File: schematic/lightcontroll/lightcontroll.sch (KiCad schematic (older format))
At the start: 0 parts

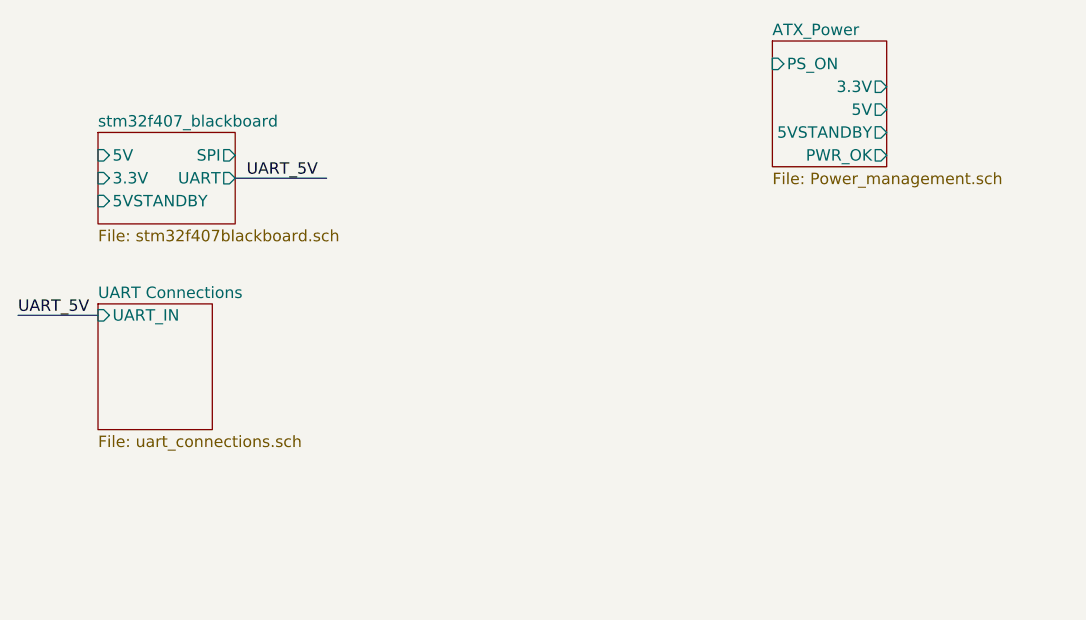
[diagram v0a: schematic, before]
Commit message: build backup
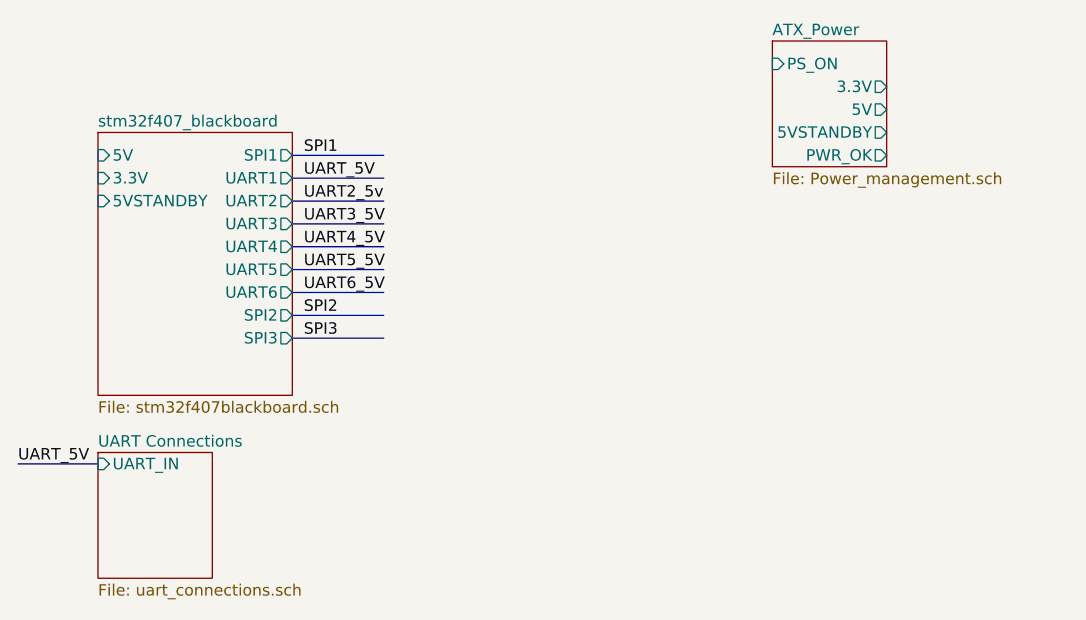
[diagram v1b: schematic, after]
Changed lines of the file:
@@
 $EndDescr
 $Sheet
-S 1600 1350 600  400
+S 1600 1350 850  1150
 U 5C818DF2
 F0 "stm32f407_blackboard" 50
@@
 F3 "3.3V" I L 1600 1550 50
 F4 "5VSTANDBY" I L 1600 1650 50
-F5 "SPI" O R 2200 1450 50
-F6 "UART" O R 2200 1550 50
+F5 "SPI1" O R 2450 1450 50
+F6 "UART1" O R 2450 1550 50
+F7 "UART2" O R 2450 1650 50
+F8 "UART3" O R 2450 1750 50
+F9 "UART4" O R 2450 1850 50
+F10 "UART5" O R 2450 1950 50
+F11 "UART6" O R 2450 2050 50
+F12 "SPI2" O R 2450 2150 50
+F13 "SPI3" O R 2450 2250 50
 $EndSheet
 $Sheet
@@
 $EndSheet
 $Sheet
-S 1600 2100 500  550
+S 1600 2750 500  550
 U 5C906D74
 F0 "UART Connections" 50
 F1 "uart_connections.sch" 50
-F2 "UART_IN" I L 1600 2150 50
+F2 "UART_IN" I L 1600 2800 50
 $EndSheet
-Text Label 2250 1550 0    50   ~ 0
+Text Label 2500 1550 0    50   ~ 0
 UART_5V
-Text Label 1250 2150 0    50   ~ 0
+Text Label 1250 2800 0    50   ~ 0
 UART_5V
 Wire Bus Line
-	2200 1550 2600 1550
+	1250 2800 1600 2800
 Wire Bus Line
-	1250 2150 1600 2150
+	2450 1550 2850 1550
+Text Label 2500 1650 0    50   ~ 0
+UART2_5v
+Text Label 2500 1750 0    50   ~ 0
+UART3_5V
+Text Label 2500 1850 0    50   ~ 0
+UART4_5V
+Text Label 2500 1950 0    50   ~ 0
+UART5_5V
+Text Label 2500 2050 0    50   ~ 0
+UART6_5V
+Text Label 2500 2150 0    50   ~ 0
+SPI2
+Text Label 2500 2250 0    50   ~ 0
+SPI3
+Text Label 2500 1450 0    50   ~ 0
+SPI1
+Wire Bus Line
+	2450 1450 2850 1450
+Wire Bus Line
+	2450 1650 2850 1650
+Wire Bus Line
+	2450 1750 2850 1750
+Wire Bus Line
+	2450 1850 2850 1850
+Wire Bus Line
+	2450 1950 2850 1950
+Wire Bus Line
+	2450 2050 2850 2050
+Wire Bus Line
+	2450 2150 2850 2150
+Wire Bus Line
+	2450 2250 2850 2250
 $EndSCHEMATC
